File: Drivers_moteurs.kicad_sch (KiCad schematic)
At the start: 12 parts, among them J15 Conn_01x02_Socket, J16 Conn_01x02_Socket, J17 Conn_01x02_Socket, J18 Conn_01x02_Socket, J19 Conn_01x02_Socket, J20 Conn_01x02_Socket

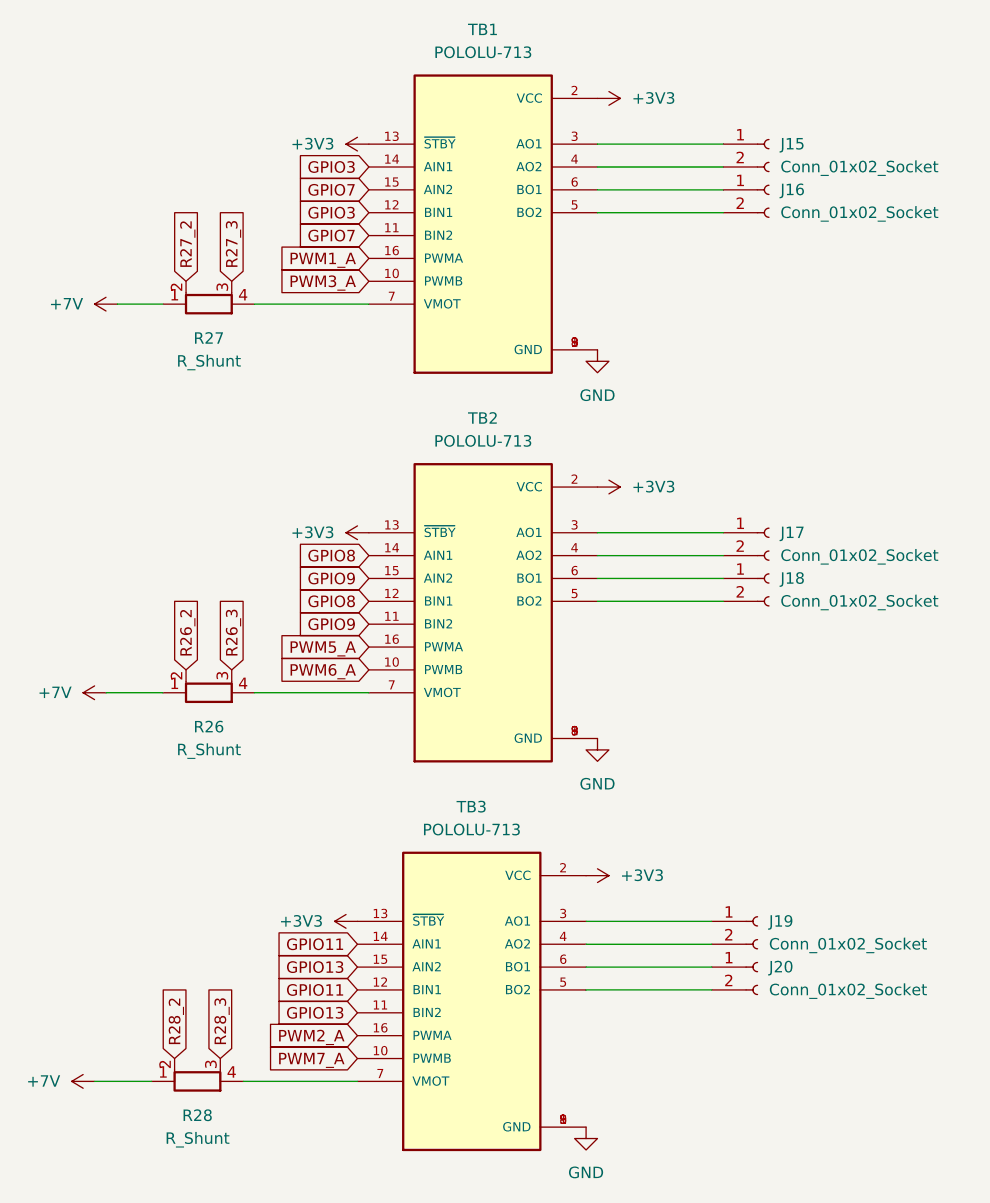
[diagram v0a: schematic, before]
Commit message: V1GD
V1 20/10/25
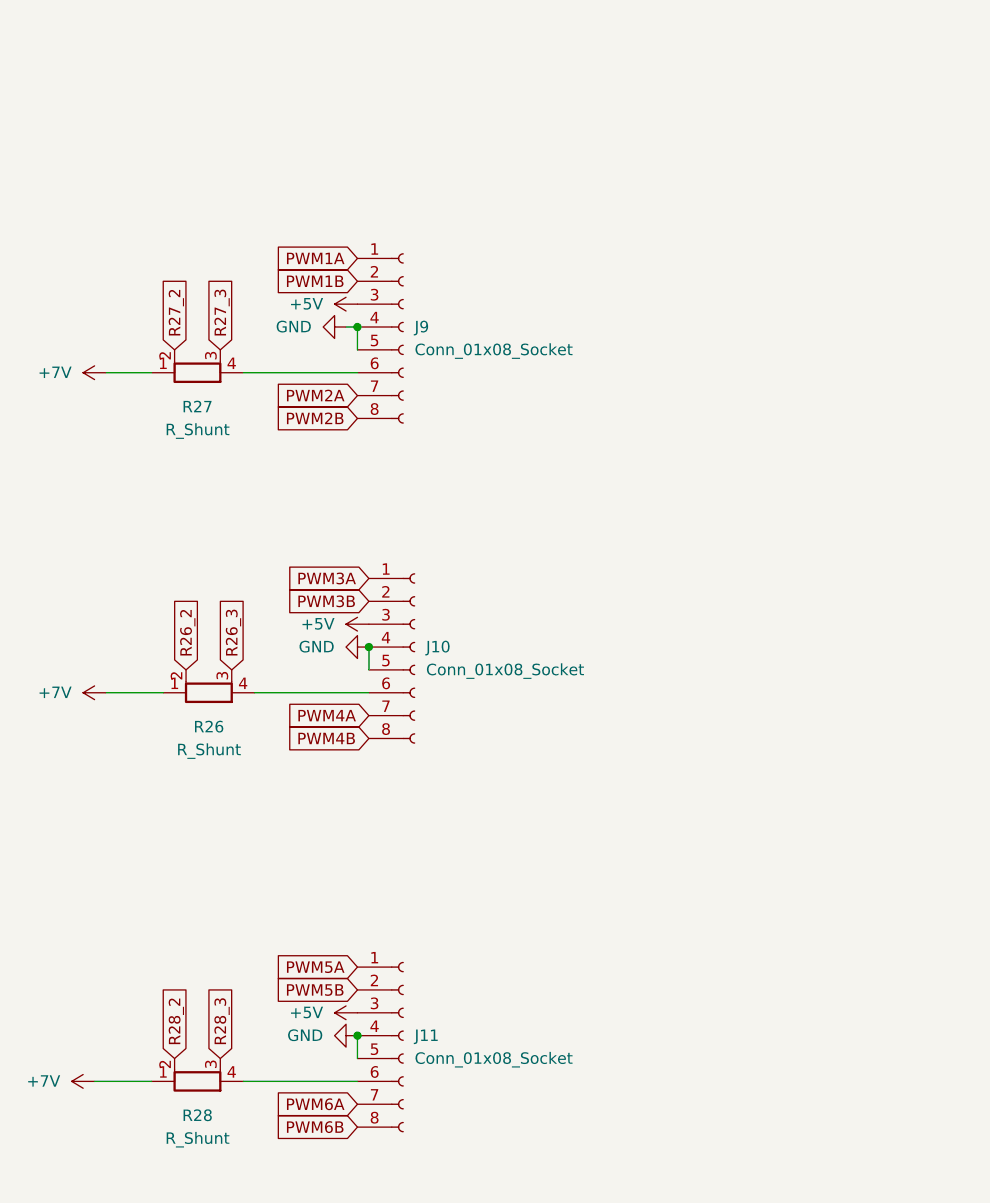
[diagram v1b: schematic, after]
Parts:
- removed J15, J16, J17, J18, J19, J20: Conn_01x02_Socket, Connector_JST:JST_EH_B2B-EH-A_1x02_P2.50mm_Vertical, symbol Connector:Conn_01x02_Socket
- removed TB1, TB2, TB3: POLOLU-713, POLOLU-713:SHIELD_POLOLU-713, symbol POLOLU-713:POLOLU-713
- added J10, J11, J9: Conn_01x08_Socket, Connector_PinHeader_2.54mm:PinHeader_1x08_P2.54mm_Vertical, symbol Connector:Conn_01x08_Socket
- R26, R27, R28: footprint (none) -> Resistor_SMD:R_1206_3216Metric
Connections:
- net GND: now also J10.4 (Pin_4), J10.5 (Pin_5), J11.4 (Pin_4), J11.5 (Pin_5), J9.4 (Pin_4), J9.5 (Pin_5)
- net at R27.4: now also J9.6 (Pin_6)
- net at R26.4: now also J10.6 (Pin_6)
- net at R28.4: now also J11.6 (Pin_6)
- new net +5V: J10.3 (Pin_3), J11.3 (Pin_3), J9.3 (Pin_3)
- new net PWM1A: J9.1 (Pin_1)
- new net PWM1B: J9.2 (Pin_2)
- new net PWM2A: J9.7 (Pin_7)
- new net PWM2B: J9.8 (Pin_8)
- new net PWM3A: J10.1 (Pin_1)
- new net PWM3B: J10.2 (Pin_2)
- new net PWM4A: J10.7 (Pin_7)
- new net PWM4B: J10.8 (Pin_8)
- new net PWM5A: J11.1 (Pin_1)
- new net PWM5B: J11.2 (Pin_2)
- new net PWM6A: J11.7 (Pin_7)
- new net PWM6B: J11.8 (Pin_8)
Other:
- moved on the sheet: R27
